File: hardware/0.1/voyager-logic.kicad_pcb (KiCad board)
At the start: 6 copper layers, 50 x 50 mm, 159 parts, among them J201 USB_C_Receptacle, J401 UART, J402 JTAG, J501 Probe, J502 Probe, SW401 KMR2, U201 USBLC6-2P6, U202 HD3SS3220, U203 TPD4EUSB30, U204 TPD4EUSB30, U301 CYUSB3014-BZXx, U302 M24M02, U501 SN74LVC245A, U502 SN74LVC245A, U701 TLV62569DRLR, U703 TLV62569DRLR, U704 TLV62569DRLR, Y301 19.2MHz

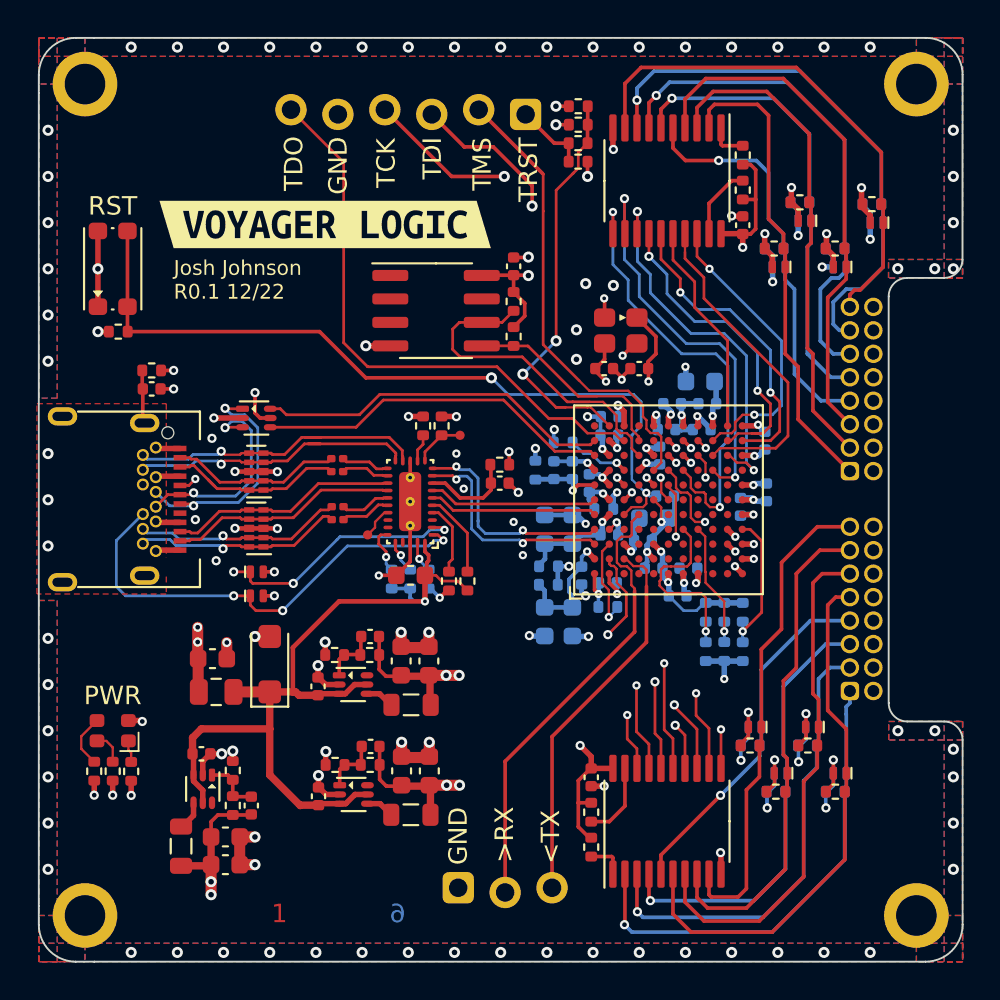
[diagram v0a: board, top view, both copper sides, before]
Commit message: clean up everything but usb3
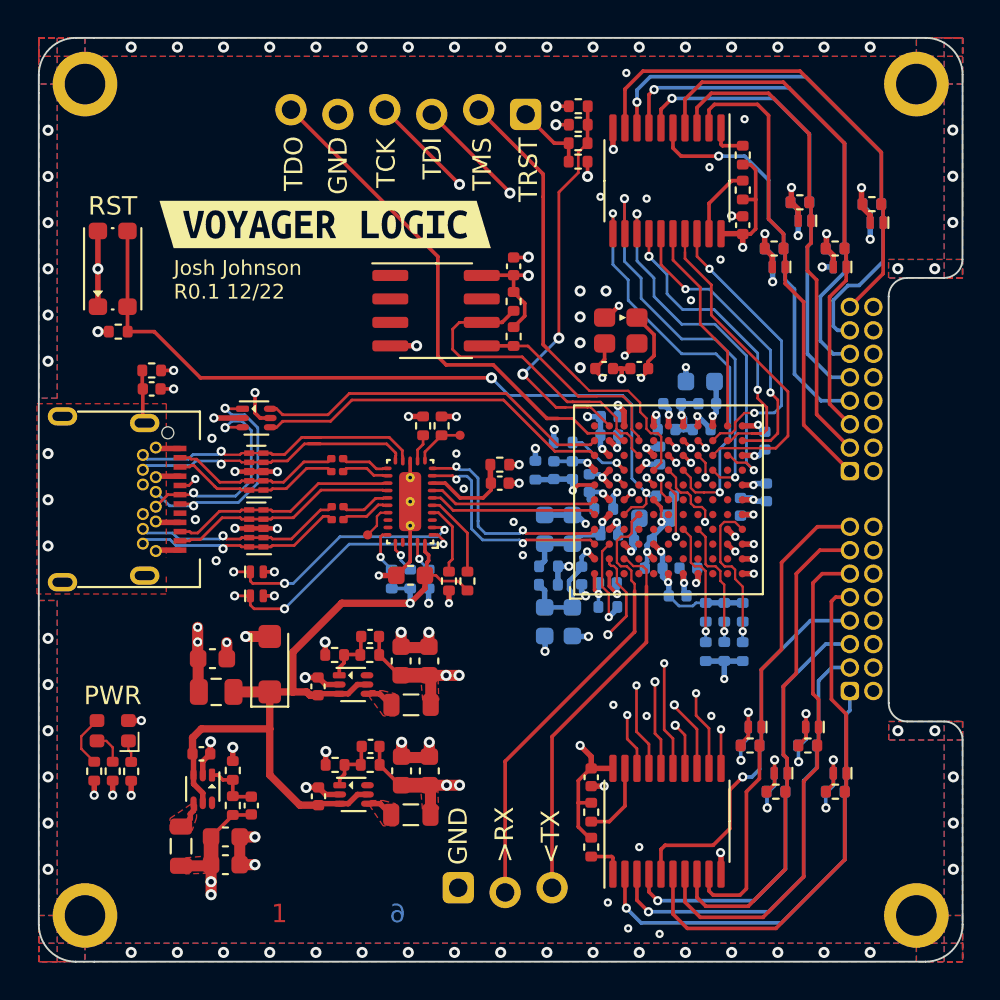
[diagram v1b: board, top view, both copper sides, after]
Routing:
- net /FX3 Logic Inputs/PMODE0: track 11.5 -> 8.44 mm
- net +3V3: track 27.8 -> 30.0 mm
- net /Debug/JTAG_TDO: track 31.2 -> 29.1 mm
- net /Power/AVDD: track 5.96 -> 3.94 mm
- net /Logic Front End/CHANNEL_3: track 19.2 -> 21.0 mm
- net GND: track 131.1 -> 132.7 mm, vias 155 -> 169
- net /FX3 Logic Inputs/CH_15: track 24.4 -> 22.9 mm
- net /FX3 Logic Inputs/PMODE2: track 8.85 -> 10.1 mm
- net +5V: track 70.4 -> 69.4 mm
- net /Logic Front End/CHANNEL_0: track 25.7 -> 24.7 mm
- net +1V2: track 33.1 -> 32.2 mm
- net /Debug/JTAG_TCK: track 31.7 -> 32.5 mm
- net /Debug/FX3_NRST: track 42.9 -> 42.1 mm
- net /Logic Front End/CHANNEL_1: track 25.1 -> 24.4 mm
- net /Logic Front End/CHANNEL_15: track 27.7 -> 27.2 mm
- added copper zone on F.Cu, net +1V2
- added copper zone on F.Cu, net +3V3
- added copper zone on F.Cu, net Net-(L701-Pad1)
- added copper zone on F.Cu, net Net-(L702-Pad1)
- added copper zone on F.Cu, net Net-(L703-Pad1)
- added copper zone on F.Cu, net VIO

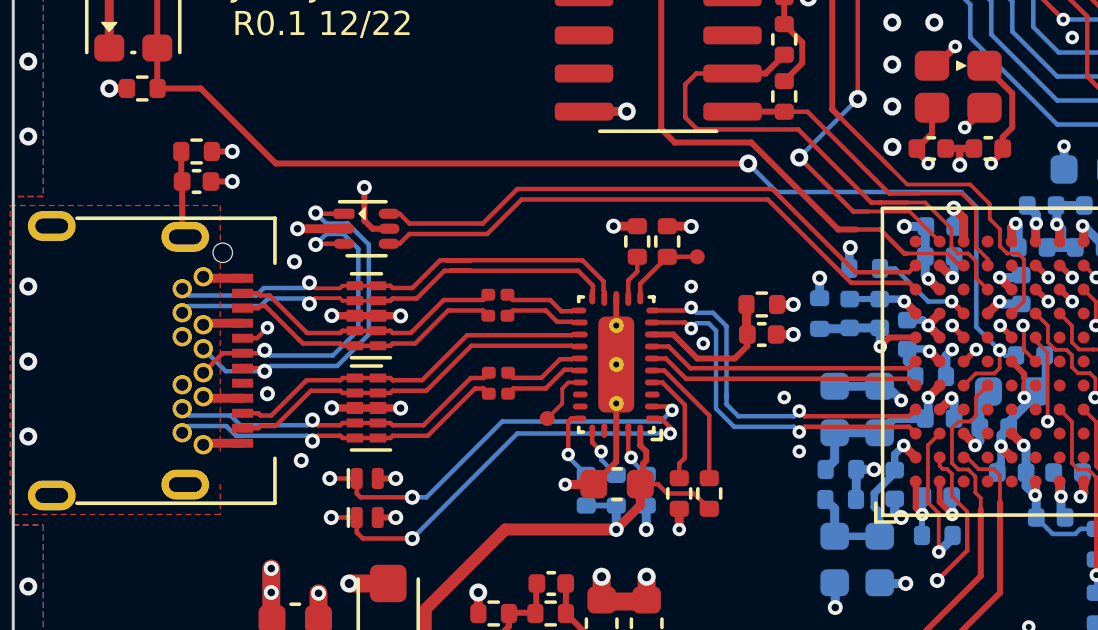
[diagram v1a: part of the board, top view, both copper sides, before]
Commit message: usb 3 clean up
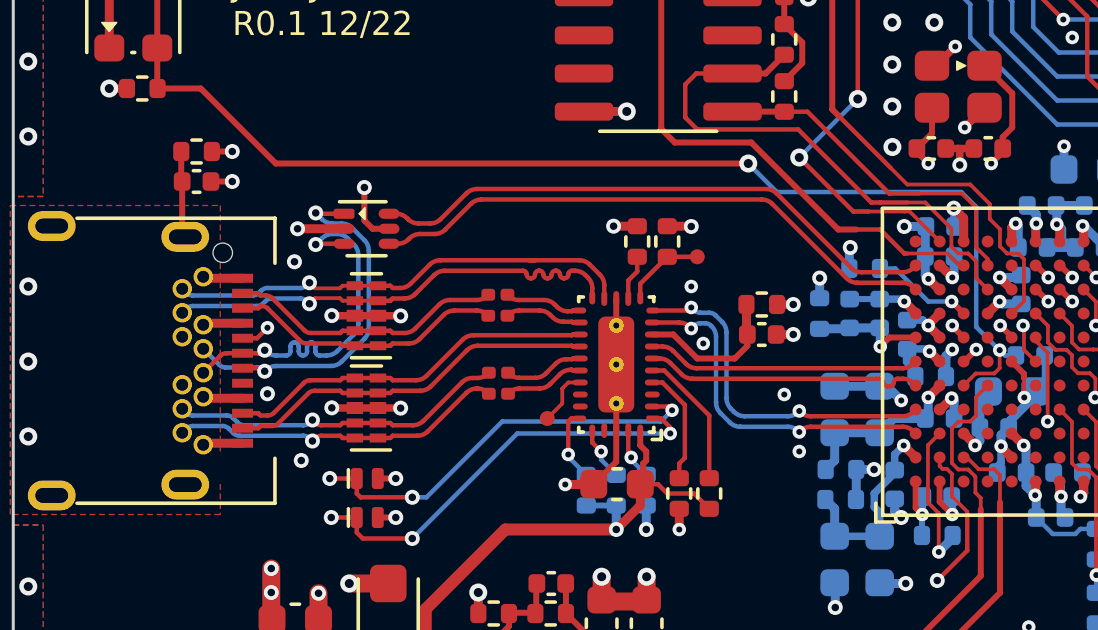
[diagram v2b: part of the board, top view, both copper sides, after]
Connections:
- net /USB C Connector/RX1N renamed /USB C Connector/RX1_N
- net /USB C Connector/RX1P renamed /USB C Connector/RX1_P
- net /USB C Connector/RX2N renamed /USB C Connector/RX2_N
- net /USB C Connector/RX2P renamed /USB C Connector/RX2_P
- net /USB C Connector/TX1N renamed /USB C Connector/TX1_N
- net /USB C Connector/TX1P renamed /USB C Connector/TX1_P
- net /USB C Connector/TX2N renamed /USB C Connector/TX2_N
- net /USB C Connector/TX2P renamed /USB C Connector/TX2_P
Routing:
- net /USB C Connector/USBD+: track 11.3 -> 12.6 mm
- net /USB C Connector/RX1_N: track 16.5 -> 15.8 mm
